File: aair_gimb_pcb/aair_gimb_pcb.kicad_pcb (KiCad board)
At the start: 2 copper layers, 6 parts, among them SW1 SW_Push, SW2 SW_Push, U1 STM32F405RGTx, X1 8MHz

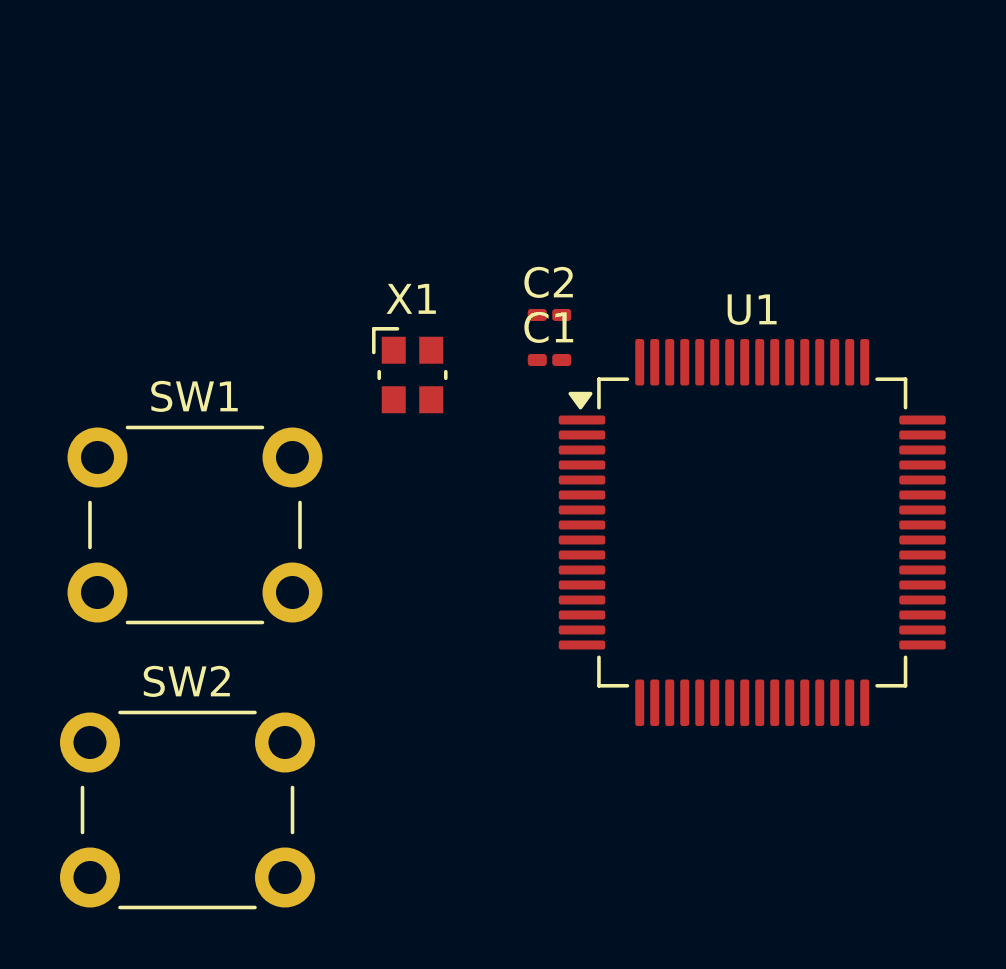
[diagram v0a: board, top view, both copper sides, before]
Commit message: mac update
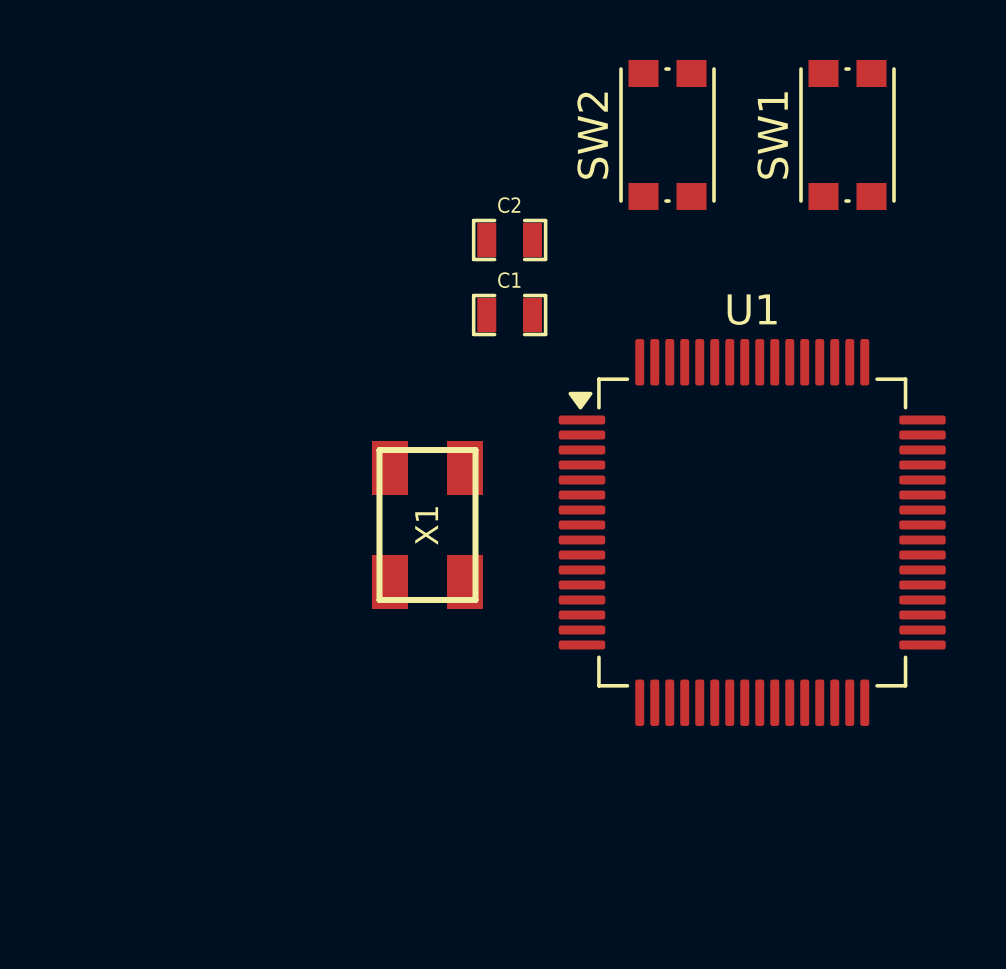
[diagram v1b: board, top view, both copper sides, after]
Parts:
- C1, C2: footprint Capacitor_SMD:C_0201_0603Metric_Pad0.64x0.40mm_HandSolder -> CRF1:SMD-0603_c
- SW1, SW2: footprint Button_Switch_THT:SW_PUSH_6mm_H5mm -> Button_Switch_SMD:SW_Push_1P1T_NO_CK_KMR2
- X1: footprint Crystal:Crystal_SMD_Abracon_ABM10-4Pin_2.5x2.0mm -> CRF1:Crystal_5x3mm
- moved SW2 27.9 mm to (87.0, 68.0), turned to 90 degrees
- moved SW1 27.2 mm to (93.0, 68.0), turned to 90 degrees
- moved X1 5.02 mm to (79.0, 81.0), turned to -90 degrees
- moved C2 2.83 mm to (81.7, 71.5)
- moved C1 2.00 mm to (81.7, 74.0)
